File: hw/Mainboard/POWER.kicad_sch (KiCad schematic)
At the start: 64 parts, among them J1 9V POWER, J2 9V POWER, J3 PET POWER, J4 5V PWR, U3 LM317AG-TN3-R, U4 XL1509-5.0E1, U5 LM317AG-TN3-R, U6 AMS1117-3.3

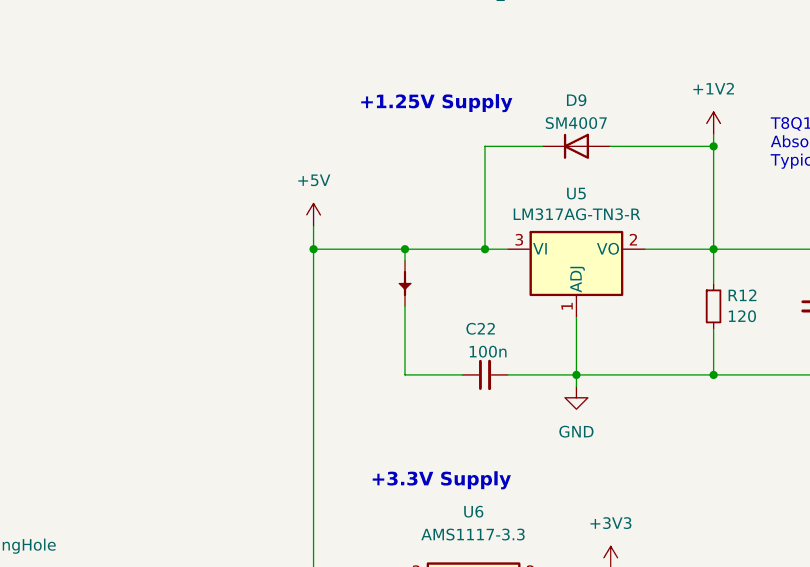
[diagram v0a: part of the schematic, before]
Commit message: hw: touch ups (wip)
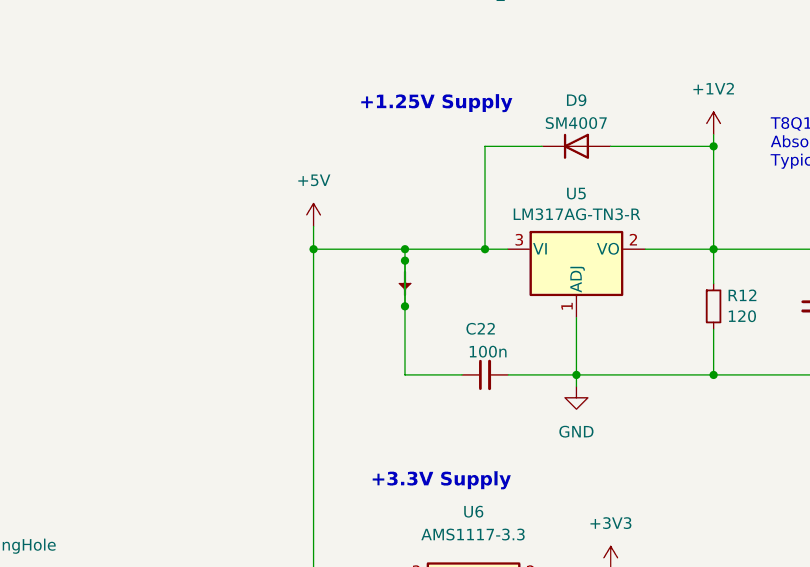
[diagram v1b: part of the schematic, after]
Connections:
- net +5V: now also C22.1, PT12.2
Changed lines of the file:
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@@
   (junction (at 63.5 36.83) (diameter 0) (color 0 0 0 0)
+  )
+  (junction (at 124.46 147.32) (diameter 0) (color 0 0 0 0)
+  )
+  (junction (at 124.46 142.24) (diameter 0) (color 0 0 0 0)
   )
   (junction (at 49.53 67.31) (diameter 0) (color 0 0 0 0)
@@
     (stroke (width 0) (type default) (color 0 0 0 0))
   )
+  (wire (pts (xy 124.46 142.24) (xy 124.46 147.32))
+    (stroke (width 0) (type default) (color 0 0 0 0))
+  )

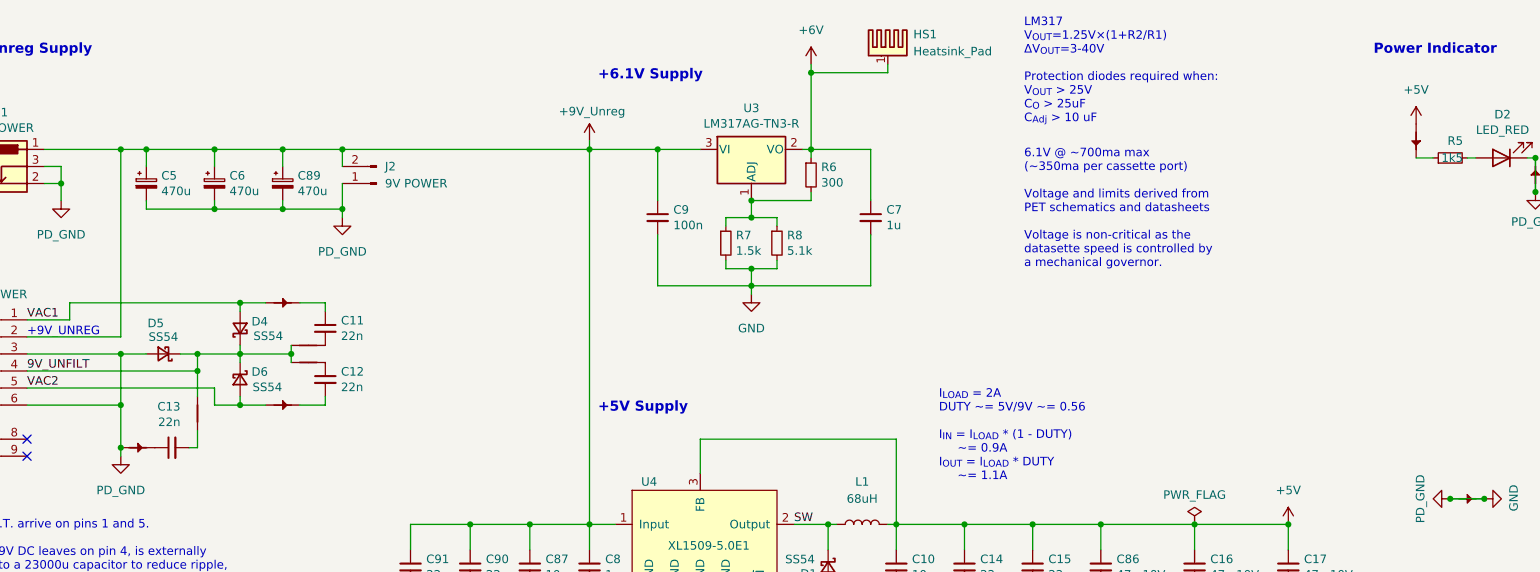
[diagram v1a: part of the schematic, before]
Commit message: hw: touchups (wip)
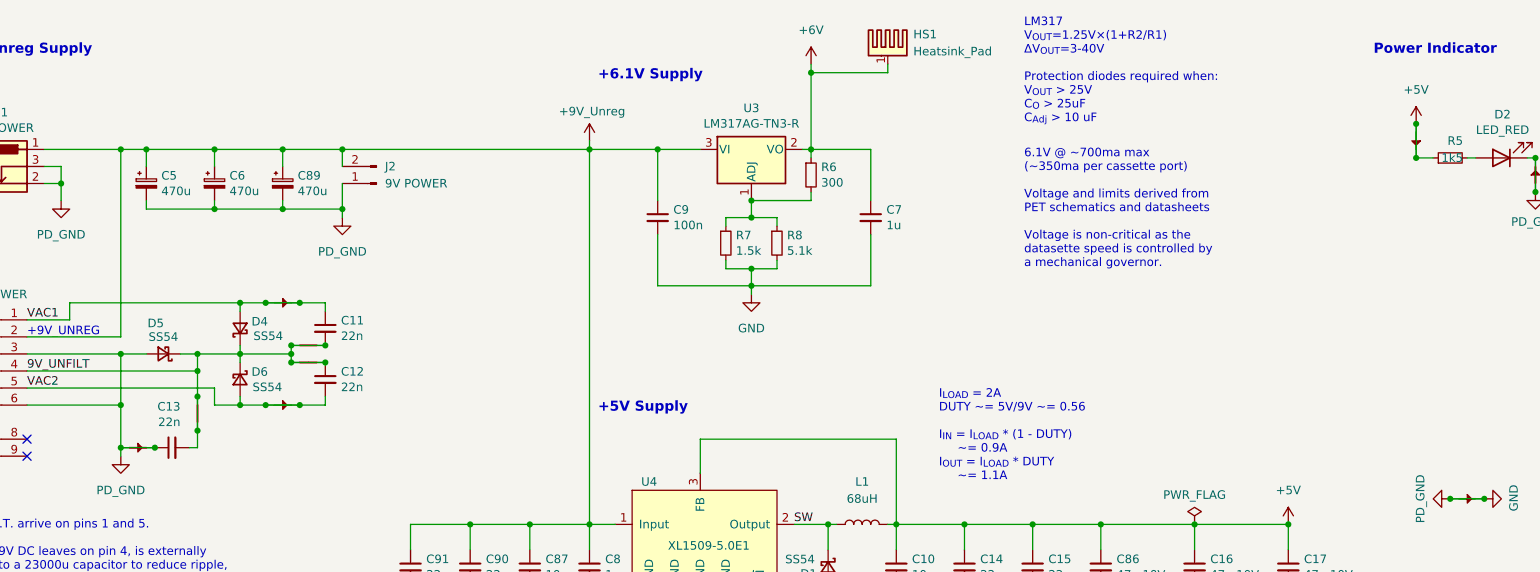
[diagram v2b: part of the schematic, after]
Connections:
- net +5V: now also PT2.2, R5.1
- net 9V_UNFILT: now also C11.2, C12.1, C13.2, PT6.2, PT7.2, PT9.2
- net GND: now also C13.1, PT10.2
- net VAC1: now also C11.1, PT5.2
- net VAC2: now also C12.2, PT8.2
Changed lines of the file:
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@@
   (junction (at 82.55 36.83) (diameter 0) (color 0 0 0 0)
   )
+  (junction (at 74.93 68.58) (diameter 0) (color 0 0 0 0)
+  )
   (junction (at 114.3 177.8) (diameter 0) (color 0 0 0 0)
   )
+  (junction (at 242.57 33.02) (diameter 0) (color 0 0 0 0)
+  )
   (junction (at 195.58 154.94) (diameter 0) (color 0 0 0 0)
   )
@@
   (junction (at 82.55 45.72) (diameter 0) (color 0 0 0 0)
   )
+  (junction (at 60.96 78.74) (diameter 0) (color 0 0 0 0)
+  )
+  (junction (at 76.2 59.69) (diameter 0) (color 0 0 0 0)
+  )
   (junction (at 261.62 138.43) (diameter 0) (color 0 0 0 0)
   )
@@
   (junction (at 195.58 106.68) (diameter 0) (color 0 0 0 0)
   )
+  (junction (at 80.01 68.58) (diameter 0) (color 0 0 0 0)
+  )
   (junction (at 209.55 92.71) (diameter 0) (color 0 0 0 0)
   )
@@
   (junction (at 223.52 92.71) (diameter 0) (color 0 0 0 0)
   )
+  (junction (at 71.12 59.69) (diameter 0) (color 0 0 0 0)
+  )
   (junction (at 110.49 106.68) (diameter 0) (color 0 0 0 0)
   )
@@
   (junction (at 73.66 45.72) (diameter 0) (color 0 0 0 0)
   )
+  (junction (at 76.2 74.93) (diameter 0) (color 0 0 0 0)
+  )
   (junction (at 73.66 36.83) (diameter 0) (color 0 0 0 0)
   )
@@
   (junction (at 195.58 140.97) (diameter 0) (color 0 0 0 0)
   )
+  (junction (at 242.57 38.1) (diameter 0) (color 0 0 0 0)
+  )
   (junction (at 165.1 92.71) (diameter 0) (color 0 0 0 0)
   )
@@
   (junction (at 147.32 177.8) (diameter 0) (color 0 0 0 0)
   )
+  (junction (at 60.96 73.66) (diameter 0) (color 0 0 0 0)
+  )
   (junction (at 132.08 186.69) (diameter 0) (color 0 0 0 0)
   )
@@
   (junction (at 114.3 140.97) (diameter 0) (color 0 0 0 0)
   )
+  (junction (at 54.61 81.28) (diameter 0) (color 0 0 0 0)
+  )
   (junction (at 175.26 92.71) (diameter 0) (color 0 0 0 0)
   )
   (junction (at 260.35 43.18) (diameter 0) (color 0 0 0 0)
   )
+  (junction (at 74.93 66.04) (diameter 0) (color 0 0 0 0)
+  )
   (junction (at 143.51 54.61) (diameter 0) (color 0 0 0 0)
   )
+  (junction (at 80.01 66.04) (diameter 0) (color 0 0 0 0)
+  )
   (junction (at 158.75 140.97) (diameter 0) (color 0 0 0 0)
   )
@@
   )
   (junction (at 195.58 92.71) (diameter 0) (color 0 0 0 0)
+  )
+  (junction (at 71.12 74.93) (diameter 0) (color 0 0 0 0)
   )
   (no_connect (at 35.56 80.01))
@@
     (stroke (width 0) (type default) (color 0 0 0 0))
   )
+  (wire (pts (xy 74.93 66.04) (xy 80.01 66.04))
+    (stroke (width 0) (type default) (color 0 0 0 0))
+  )
   (wire (pts (xy 124.46 147.32) (xy 124.46 154.94))
     (stroke (width 0) (type default) (color 0 0 0 0))
@@
     (stroke (width 0) (type default) (color 0 0 0 0))
   )
+  (wire (pts (xy 74.93 68.58) (xy 80.01 68.58))
+    (stroke (width 0) (type default) (color 0 0 0 0))
+  )
   (wire (pts (xy 246.38 151.13) (xy 246.38 143.51))
     (stroke (width 0) (type default) (color 0 0 0 0))
@@
     (stroke (width 0) (type default) (color 0 0 0 0))
   )
+  (wire (pts (xy 60.96 73.66) (xy 60.96 78.74))
+    (stroke (width 0) (type default) (color 0 0 0 0))
+  )
   (wire (pts (xy 195.58 101.6) (xy 195.58 106.68))
     (stroke (width 0) (type default) (color 0 0 0 0))
@@
     (stroke (width 0) (type default) (color 0 0 0 0))
   )
+  (wire (pts (xy 71.12 59.69) (xy 76.2 59.69))
+    (stroke (width 0) (type default) (color 0 0 0 0))
+  )
   (wire (pts (xy 223.52 92.71) (xy 223.52 96.52))
     (stroke (width 0) (type default) (color 0 0 0 0))
@@
     (stroke (width 0) (type default) (color 0 0 0 0))
   )
+  (wire (pts (xy 49.53 81.28) (xy 54.61 81.28))
+    (stroke (width 0) (type default) (color 0 0 0 0))
+  )
   (wire (pts (xy 185.42 92.71) (xy 195.58 92.71))
     (stroke (width 0) (type default) (color 0 0 0 0))
@@
     (stroke (width 0) (type default) (color 0 0 0 0))
   )
+  (wire (pts (xy 71.12 74.93) (xy 76.2 74.93))
+    (stroke (width 0) (type default) (color 0 0 0 0))
+  )
   (wire (pts (xy 135.89 80.01) (xy 135.89 85.09))
     (stroke (width 0) (type default) (color 0 0 0 0))
@@
     (stroke (width 0) (type default) (color 0 0 0 0))
   )
+  (wire (pts (xy 242.57 33.02) (xy 242.57 38.1))
+    (stroke (width 0) (type default) (color 0 0 0 0))
+  )

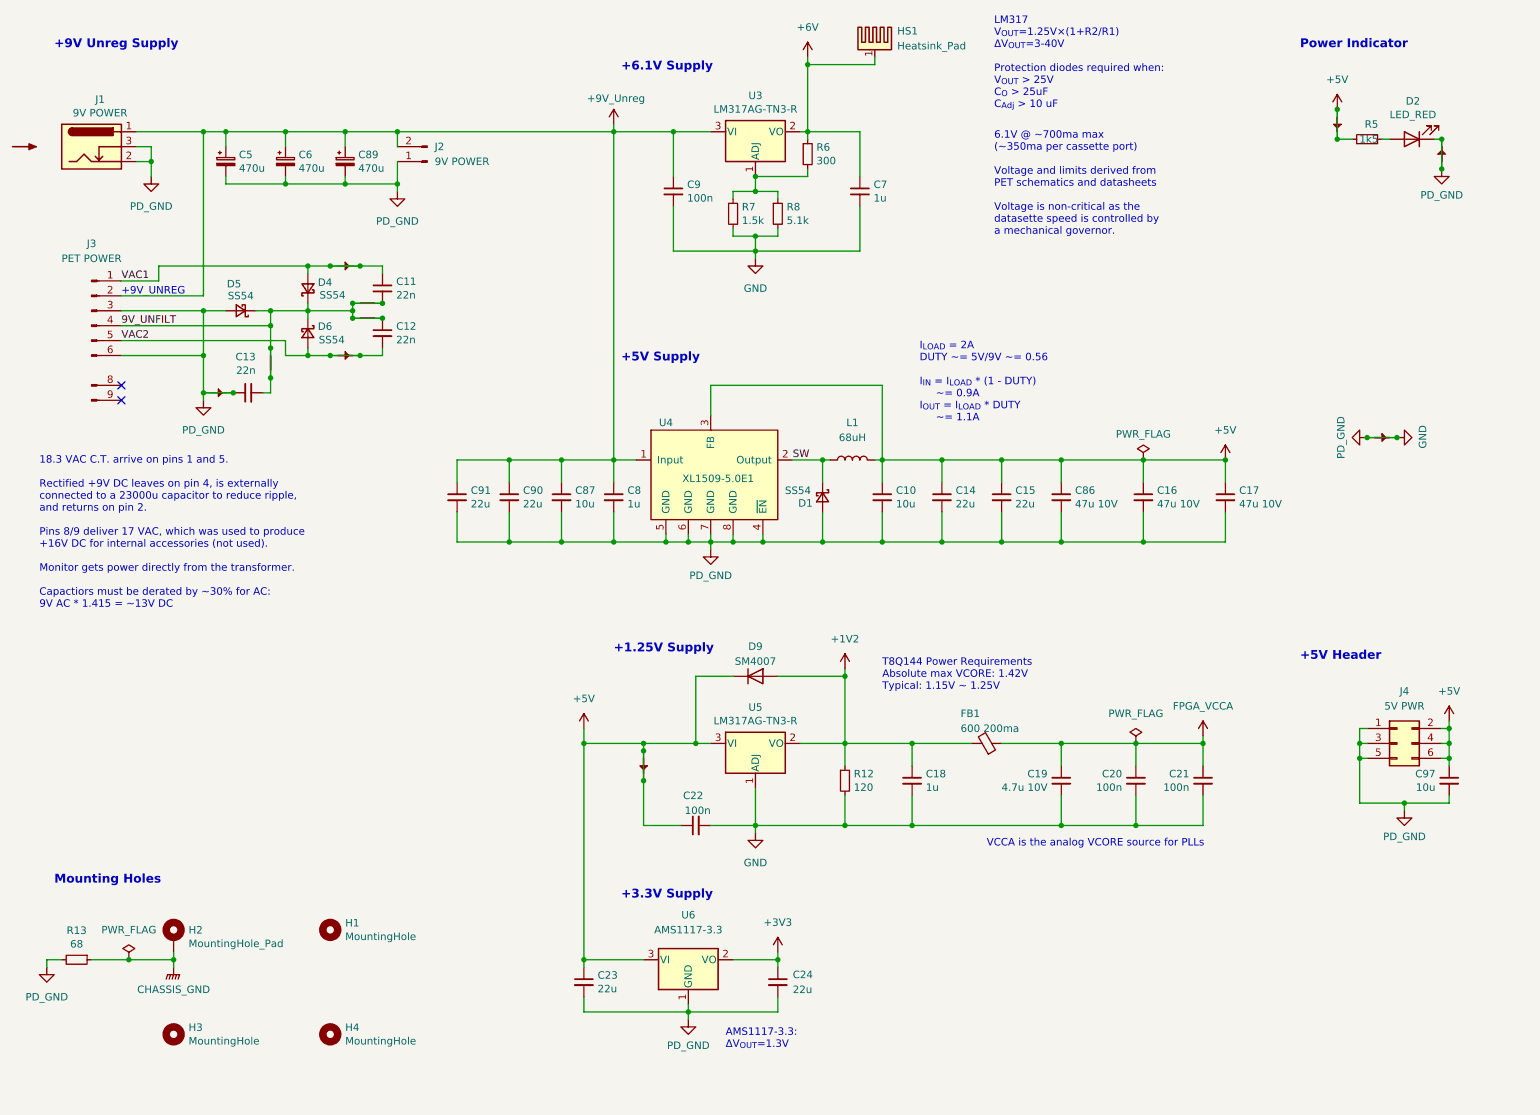
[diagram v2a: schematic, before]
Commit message: hw: caps & logos (wip)
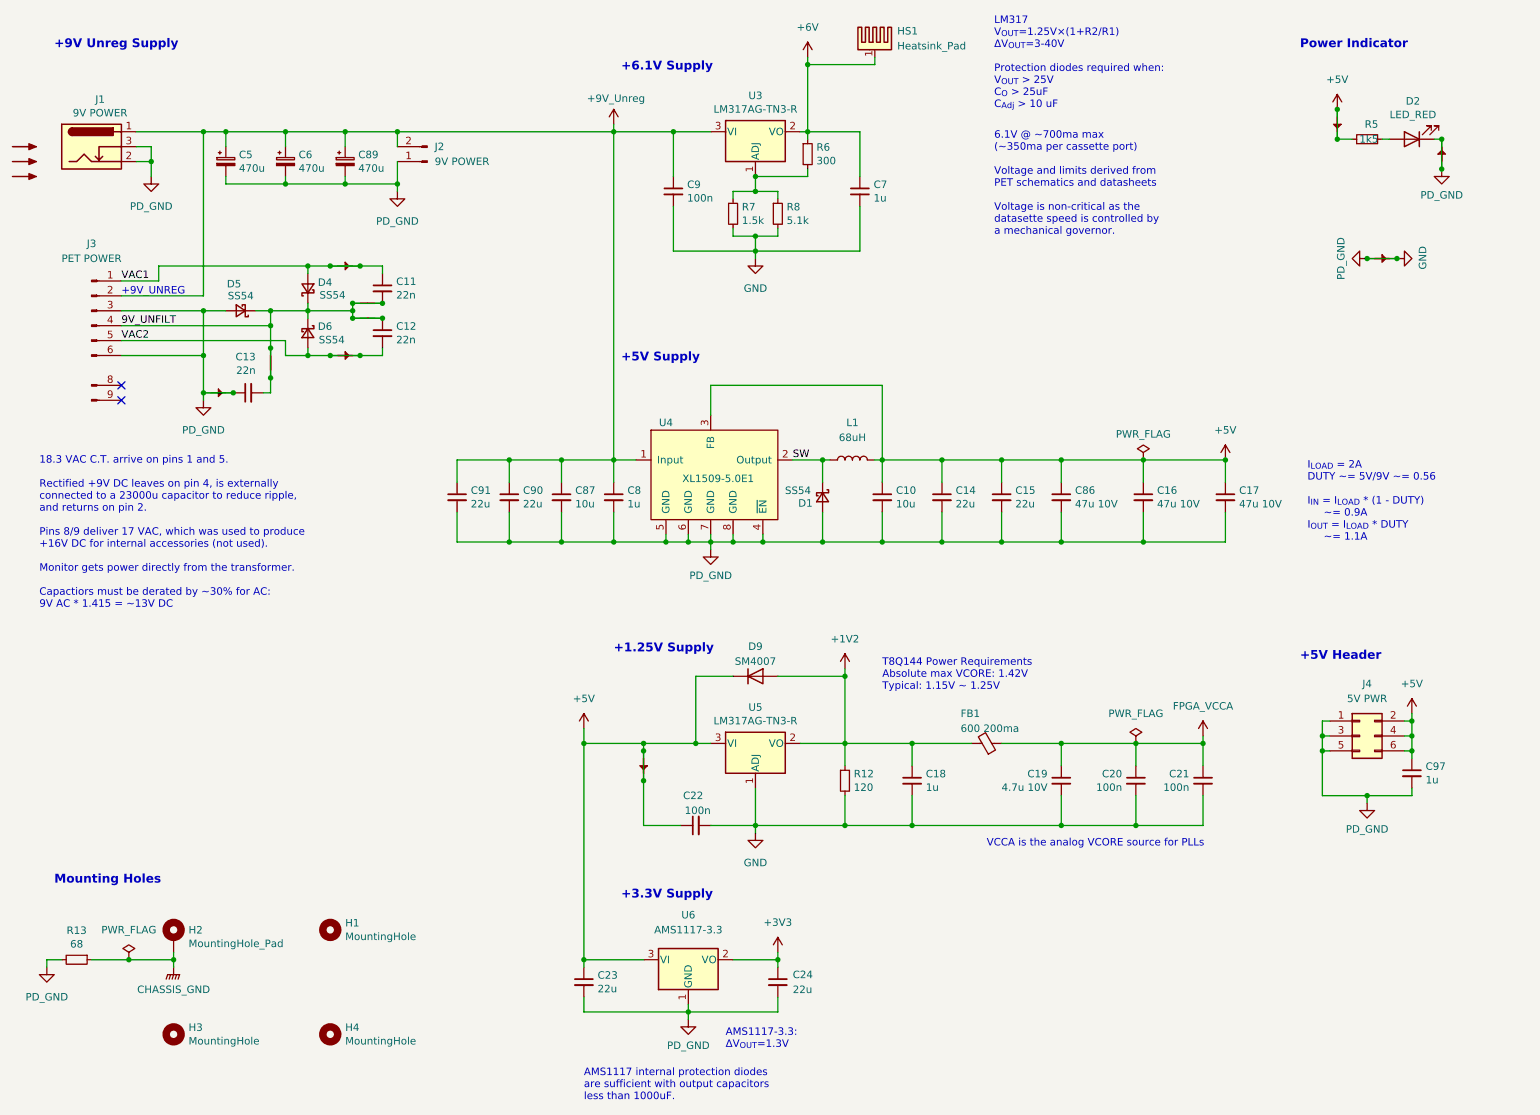
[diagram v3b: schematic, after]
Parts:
- added SYM2: SYM_Arrow_Small, PET:EconoPET_QR, symbol Graphic:SYM_Arrow_Small
- added SYM3: SYM_Arrow_Small, PET:EconoPET_Model, symbol Graphic:SYM_Arrow_Small
- C97: value 10u -> 1u; footprint Capacitor_SMD:C_0603_1608Metric -> Capacitor_SMD:C_0402_1005Metric; LCSC C96446 -> C52923
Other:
- note added: "AMS1117 internal protection diodes are sufficient with output capacitors less than 1000uF."
- title: CBM PET Mainboard Replacement -> EconoPET 40/8096
- moved on the sheet: J4
